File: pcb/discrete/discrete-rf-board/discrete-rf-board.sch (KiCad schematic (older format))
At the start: 3 parts

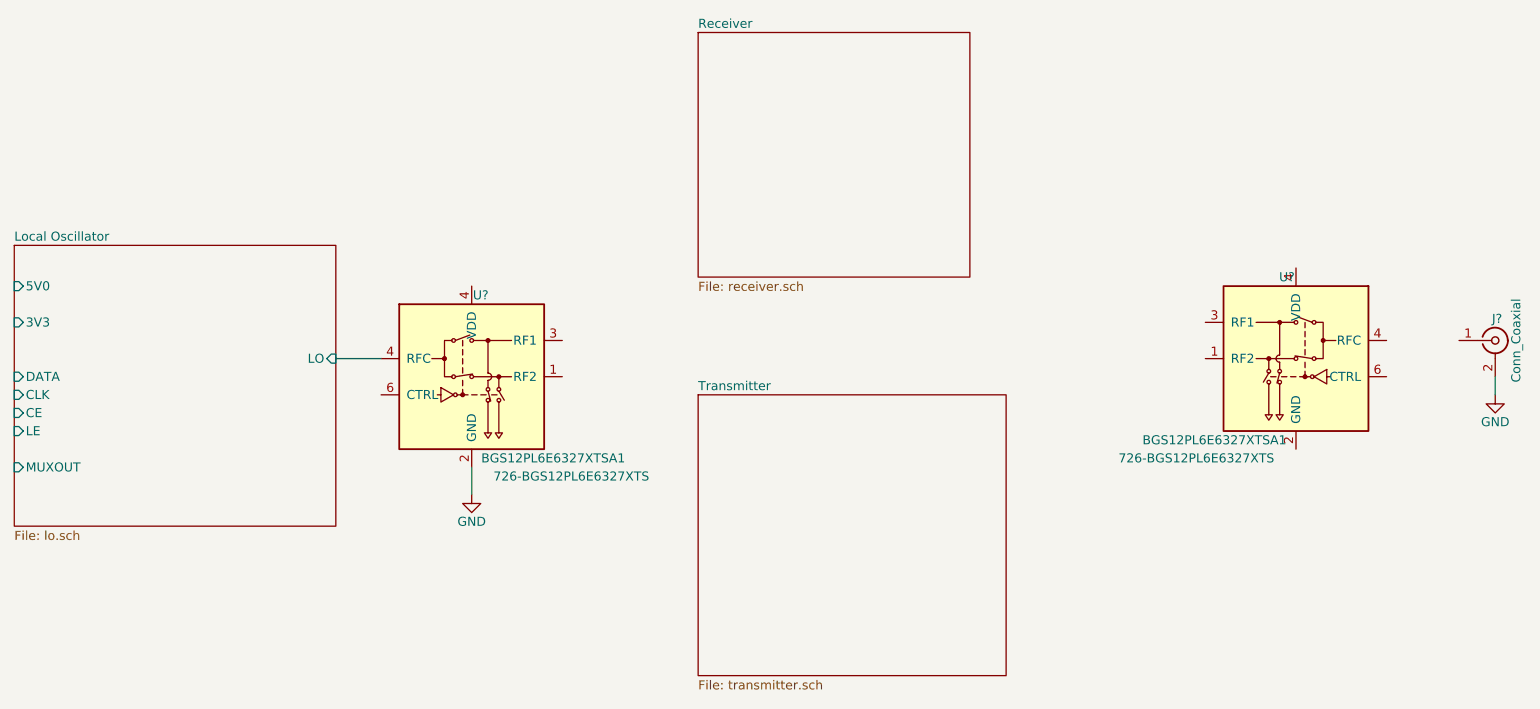
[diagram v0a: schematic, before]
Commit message: Save changes while moving over to the new laptop
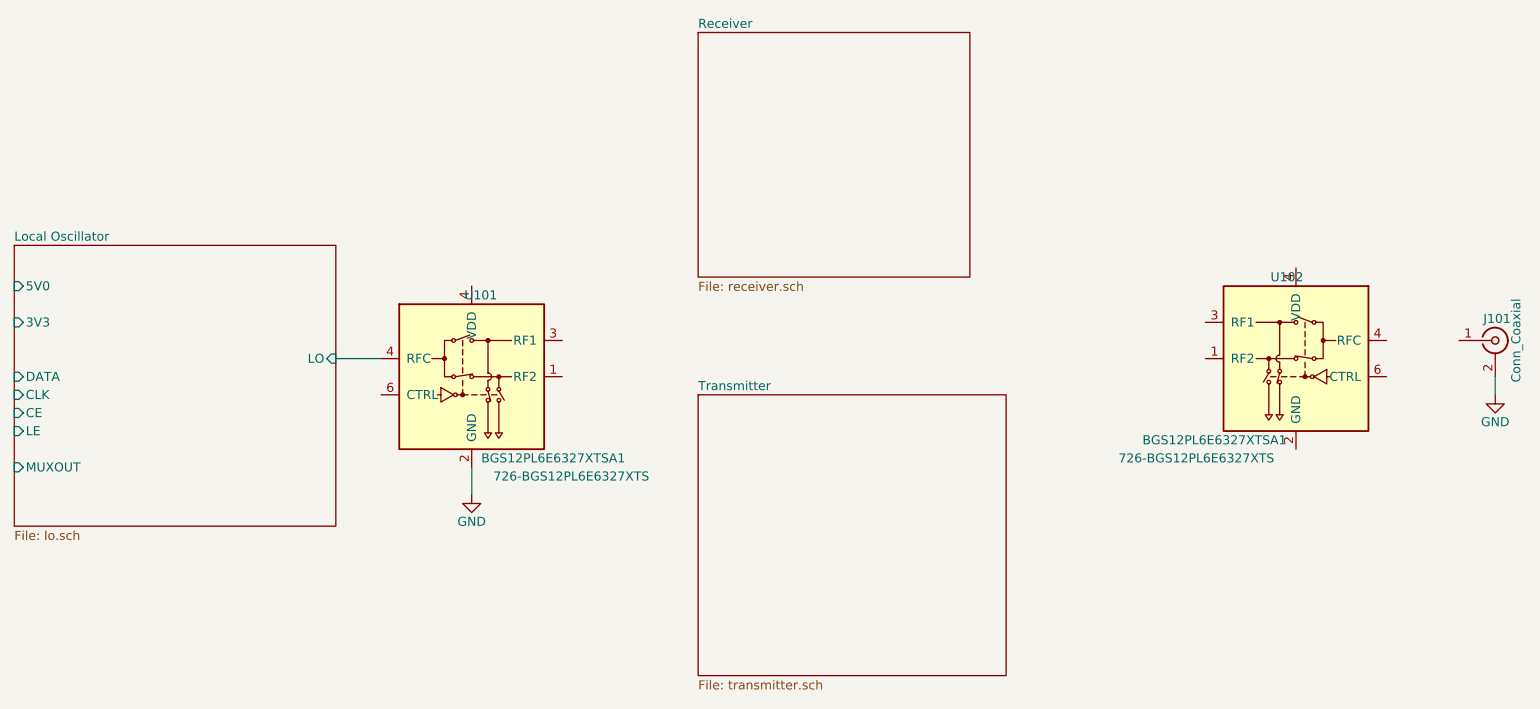
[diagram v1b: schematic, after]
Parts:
- gave numbers to parts that had none: 3
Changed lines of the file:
@@
 $Descr USLetter 11000 8500
 encoding utf-8
-Sheet 1 9
+Sheet 1 11
 Title ""
 Date ""
@@
 $EndSheet
 $Comp
-L discrete-parts:BGS12PL6E6327XTSA1 U?
+L discrete-parts:BGS12PL6E6327XTSA1 U101
 U 1 1 5CC15EED
 P 4350 3450
-F 0 "U?" H 4400 3900 50  0000 C CNN
+F 0 "U101" H 4400 3900 50  0000 C CNN
 F 1 "BGS12PL6E6327XTSA1" H 4800 3000 50  0000 C CNN
 F 2 "" H 4350 3450 50  0001 C CNN
@@
 $EndSheet
 $Comp
-L power:GND #PWR?
+L power:GND #PWR0101
 U 1 1 5CC42654
 P 4350 4100
-F 0 "#PWR?" H 4350 3850 50  0001 C CNN
+F 0 "#PWR0101" H 4350 3850 50  0001 C CNN
 F 1 "GND" H 4350 3950 50  0000 C CNN
 F 2 "" H 4350 4100 50  0001 C CNN
@@
 	4350 4100 4350 3950
 $Comp
-L discrete-parts:BGS12PL6E6327XTSA1 U?
+L discrete-parts:BGS12PL6E6327XTSA1 U102
 U 1 1 5CC42E59
 P 8900 3350
-F 0 "U?" H 8950 3800 50  0000 C CNN
+F 0 "U102" H 8950 3800 50  0000 C CNN
 F 1 "BGS12PL6E6327XTSA1" H 9350 2900 50  0000 C CNN
 F 2 "" H 8900 3350 50  0001 C CNN
@@
 $EndComp
 $Comp
-L Connector:Conn_Coaxial J?
+L Connector:Conn_Coaxial J101
 U 1 1 5CC44B33
 P 10000 3250
-F 0 "J?" H 10010 3370 50  0000 C CNN
+F 0 "J101" H 10010 3370 50  0000 C CNN
 F 1 "Conn_Coaxial" V 10115 3250 50  0000 C CNN
 F 2 "" H 10000 3250 50  0001 C CNN
@@
 $EndComp
 $Comp
-L power:GND #PWR?
+L power:GND #PWR0102
 U 1 1 5CC454AB
 P 10000 3550
-F 0 "#PWR?" H 10000 3300 50  0001 C CNN
+F 0 "#PWR0102" H 10000 3300 50  0001 C CNN
 F 1 "GND" H 10000 3400 50  0000 C CNN
 F 2 "" H 10000 3550 50  0001 C CNN
